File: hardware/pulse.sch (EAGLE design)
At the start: 17 parts, among them IC3 TLC272P, U1 ATTINY45-20PU

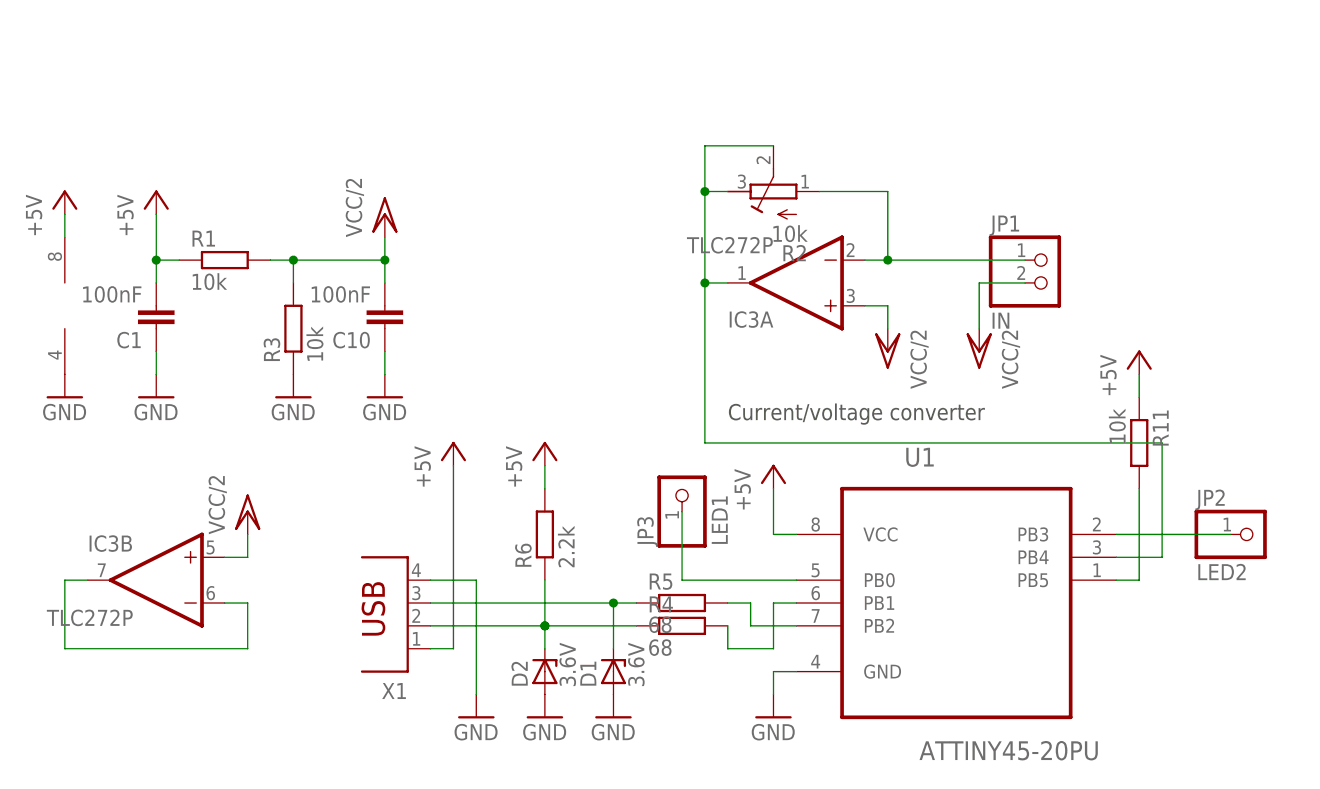
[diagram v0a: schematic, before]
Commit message: Updated schematic & board.
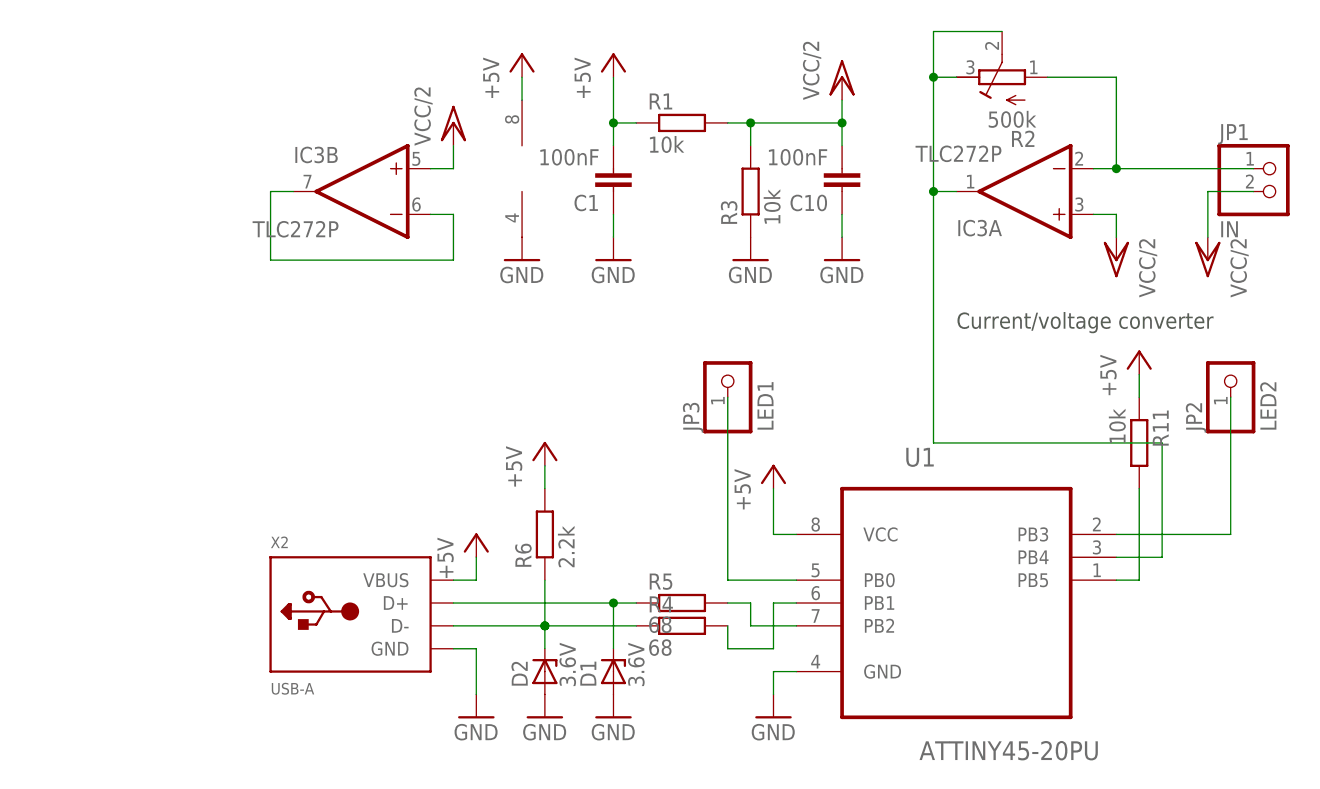
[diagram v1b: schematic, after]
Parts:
- removed X1: (no value), con-berg:PN87520
- added X2: USB-A, adafruit:USB-A
- R2: value 10k -> 500k
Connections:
- net +5V: now also X2.VBUS; no longer X1.1
- net GND: now also X2.GND; no longer X1.4
- net N$10: now also X2.D+; no longer X1.3
- net N$11: now also X2.D-; no longer X1.2
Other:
- moved on the sheet: C1, C10, IC3A, IC3B, JP1, JP2, JP3, R1, R2, R3
